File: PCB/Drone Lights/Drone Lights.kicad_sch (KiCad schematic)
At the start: 34 parts, among them J1 Proto Pin, J10 Prog_Connector, J11 Proto Pin, J12 Proto Pin, J13 Proto Pin, J14 Proto Pin, J2 Input, J3 Proto Pin, J4 Proto Pin, J5 Proto Pin, J6 Proto Pin, J7 Proto Pin, J8 Proto Pin, J9 Proto Pin, SW1 CT11024.3F160, SW2 CT11024.3F160, SW3 GF-123-0054, U1 ATTINY84A-PU

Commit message: Updated assembly guide
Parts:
- C1: Digikey No. (none) -> 445-1314-1-ND; MPN (none) -> C1608X7R1H104K080AA
- D1: Green MPN (none) -> XPEBGR-L1-0000-00F01; Red MPN (none) -> XPEBRD-L1-0000-00501; White MPN (none) -> XPEBWT-L1-0000-00C51
- D2, D3: MPN (none) -> B1911USD-20D000114U1930; Manufacturer PN B1911USD-20D000114U1930 -> (none)
- MOSFET1: Digikey No. (none) -> T2N7002BKLMCT-ND; MPN (none) -> T2N7002BK,LM
- R1: Digikey No. (none) -> P10.0HCT-ND; MPN (none) -> ERJ-3EKF10R0V
- R2, R3, R4: Digikey No. (none) -> RNCP0603FTD10K0CT-ND; MPN (none) -> RNCP0603FTD10K0
- R5: Digikey No. (none) -> 2019-RK73H1JRTTD4701FCT-ND; MPN (none) -> RK73H1JRTTD4701F
- SW1, SW2: Digikey No. (none) -> 2449-CT11024.3F160-ND; MPN (none) -> CT11024.3F160
- SW3: Digikey No. (none) -> CWI333-ND; MPN (none) -> GF-123-0054
- U1: Digikey No. (none) -> ATTINY84A-PU-ND; MPN (none) -> ATTINY84A-PU
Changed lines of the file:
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@@
+      (effects (font (size 1.27 1.27)) hide)
+    )
+    (property "Green MPN" "XPEBGR-L1-0000-00F01" (id 4) (at 35.56 74.295 0)
+      (effects (font (size 1.27 1.27)) hide)
+    )
+    (property "White MPN" "XPEBWT-L1-0000-00C51" (id 5) (at 35.56 74.295 0)
+      (effects (font (size 1.27 1.27)) hide)
+    )
+    (property "Red MPN" "XPEBRD-L1-0000-00501" (id 6) (at 35.56 74.295 0)
       (effects (font (size 1.27 1.27)) hide)
     )
@@
     )
     (property "Datasheet" "" (id 3) (at 46.99 69.215 0)
-      (effects (font (size 1.524 1.524)))
+      (effects (font (size 1.524 1.524)) hide)
+    )
+    (property "Digikey No." "T2N7002BKLMCT-ND" (id 4) (at 46.99 69.215 0)
+      (effects (font (size 1.27 1.27)) hide)
+    )
+    (property "MPN" "T2N7002BK,LM" (id 5) (at 46.99 69.215 0)
+      (effects (font (size 1.27 1.27)) hide)
     )
     (pin "1")
@@
       (effects (font (size 1.27 1.27)) hide)
     )
+    (property "Digikey No." "P10.0HCT-ND" (id 4) (at 42.545 74.295 90)
+      (effects (font (size 1.27 1.27)) hide)
+    )
+    (property "MPN" "ERJ-3EKF10R0V" (id 5) (at 42.545 74.295 90)
+      (effects (font (size 1.27 1.27)) hide)
+    )
     (pin "1")
     (pin "2")
@@
       (effects (font (size 1.27 1.27)) hide)
     )
+    (property "Digikey No." "RNCP0603FTD10K0CT-ND" (id 4) (at 218.44 66.04 90)
+      (effects (font (size 1.27 1.27)) hide)
+    )
+    (property "MPN" "RNCP0603FTD10K0" (id 5) (at 218.44 66.04 90)
+      (effects (font (size 1.27 1.27)) hide)
+    )
     (pin "1")
     (pin "2")
@@
       (effects (font (size 1.27 1.27)) hide)
     )
+    (property "Digikey No." "445-1314-1-ND" (id 4) (at 116.205 61.595 0)
+      (effects (font (size 1.27 1.27)) hide)
+    )
+    (property "MPN" "C1608X7R1H104K080AA" (id 5) (at 116.205 61.595 0)
+      (effects (font (size 1.27 1.27)) hide)
+    )
     (pin "1")
     (pin "2")
@@
     (property "Datasheet" "" (id 3) (at 46.99 121.285 0)
       (effects (font (size 1.524 1.524)))
+    )
+    (property "Digikey No." "2449-CT11024.3F160-ND" (id 4) (at 46.99 121.285 0)
+      (effects (font (size 1.27 1.27)) hide)
+    )
+    (property "MPN" "CT11024.3F160" (id 5) (at 46.99 121.285 0)
+      (effects (font (size 1.27 1.27)) hide)
     )
     (pin "1")
@@
       (effects (font (size 1.27 1.27)) hide)
     )
+    (property "Digikey No." "2019-RK73H1JRTTD4701FCT-ND" (id 4) (at 232.41 101.6 90)
+      (effects (font (size 1.27 1.27)) hide)
+    )
+    (property "MPN" "RK73H1JRTTD4701F" (id 5) (at 232.41 101.6 90)
+      (effects (font (size 1.27 1.27)) hide)
+    )
     (pin "1")
     (pin "2")
@@
       (effects (font (size 1.27 1.27)) hide)
     )
-    (property "Manufacturer PN" "B1911USD-20D000114U1930" (id 5) (at 248.92 66.04 0)
+    (property "MPN" "B1911USD-20D000114U1930" (id 5) (at 248.92 66.04 0)
       (effects (font (size 1.27 1.27)) hide)
     )
@@
       (effects (font (size 1.27 1.27)) hide)
     )
+    (property "Digikey No." "RNCP0603FTD10K0CT-ND" (id 4) (at 80.01 126.365 90)
+      (effects (font (size 1.27 1.27)) hide)
+    )
+    (property "MPN" "RNCP0603FTD10K0" (id 5) (at 80.01 126.365 90)
+      (effects (font (size 1.27 1.27)) hide)
+    )
     (pin "1")
     (pin "2")
@@
       (effects (font (size 1.27 1.27)) hide)
     )
+    (property "Digikey No." "RNCP0603FTD10K0CT-ND" (id 4) (at 80.01 109.22 90)
+      (effects (font (size 1.27 1.27)) hide)
+    )
+    (property "MPN" "RNCP0603FTD10K0" (id 5) (at 80.01 109.22 90)
+      (effects (font (size 1.27 1.27)) hide)
+    )
     (pin "1")
     (pin "2")
@@
     )
     (property "Datasheet" "" (id 3) (at 62.23 141.605 0)
-      (effects (font (size 1.524 1.524)))
+      (effects (font (size 1.524 1.524)) hide)
+    )
+    (property "Digikey No." "CWI333-ND" (id 4) (at 62.23 141.605 0)
+      (effects (font (size 1.27 1.27)) hide)
+    )
+    (property "MPN" "GF-123-0054" (id 5) (at 62.23 141.605 0)
+      (effects (font (size 1.27 1.27)) hide)
     )
     (pin "1")
@@
       (effects (font (size 1.27 1.27)) hide)
     )
-    (property "Manufacturer PN" "B1911USD-20D000114U1930" (id 5) (at 240.665 101.6 0)
+    (property "MPN" "B1911USD-20D000114U1930" (id 5) (at 240.665 101.6 0)
       (effects (font (size 1.27 1.27)) hide)
     )
@@
     )
     (property "Datasheet" "" (id 3) (at 46.99 104.14 0)
-      (effects (font (size 1.524 1.524)))
+      (effects (font (size 1.524 1.524)) hide)
+    )
+    (property "Digikey No." "2449-CT11024.3F160-ND" (id 4) (at 46.99 104.14 0)
+      (effects (font (size 1.27 1.27)) hide)
+    )
+    (property "MPN" "CT11024.3F160" (id 5) (at 46.99 104.14 0)
+      (effects (font (size 1.27 1.27)) hide)
     )
     (pin "1")
@@
       (effects (font (size 1.524 1.524)) hide)
     )
-    (property "Datasheet" "" (id 3) (at 121.92 65.405 0)
-      (effects (font (size 1.524 1.524)))
-    )
-    (pin "1")
+    (property "Datasheet" "https://www.digikey.ca/en/products/detail/microchip-technology/ATTINY84A-PU/2774082" (id 3) (at 121.92 65.405 0)
+      (effects (font (size 1.524 1.524)) hide)
+    )
+    (property "Digikey No." "ATTINY84A-PU-ND" (id 4) (at 121.92 65.405 0)
+      (effects (font (size 1.27 1.27)) hide)
+    )
+    (property "MPN" "ATTINY84A-PU" (id 5) (at 121.92 65.405 0)
+      (effects (font (size 1.27 1.27)) hide)
+    )
+    (pin "1")

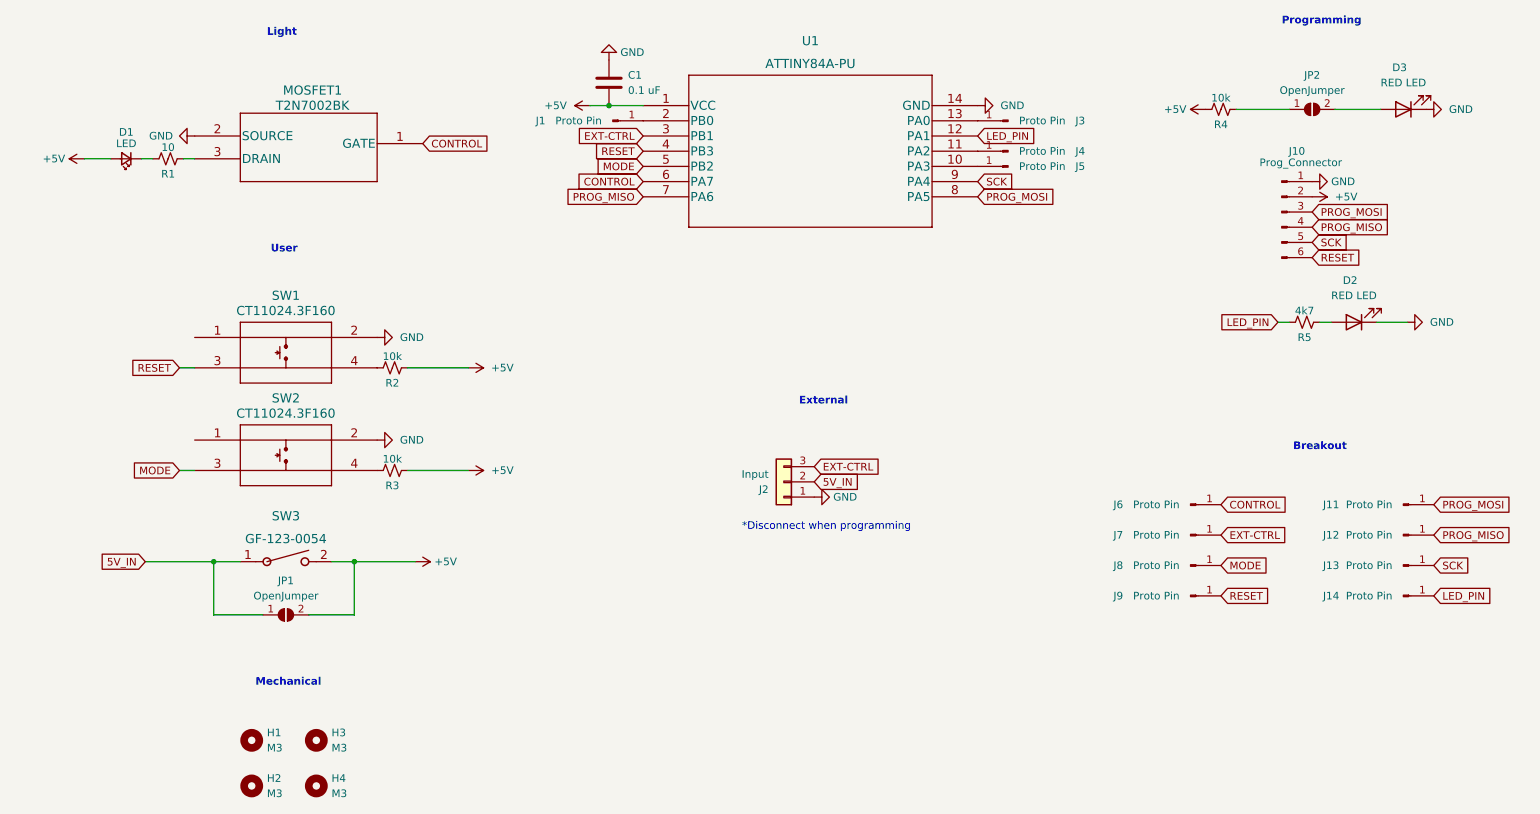
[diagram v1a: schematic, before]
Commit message: Updated with local copy
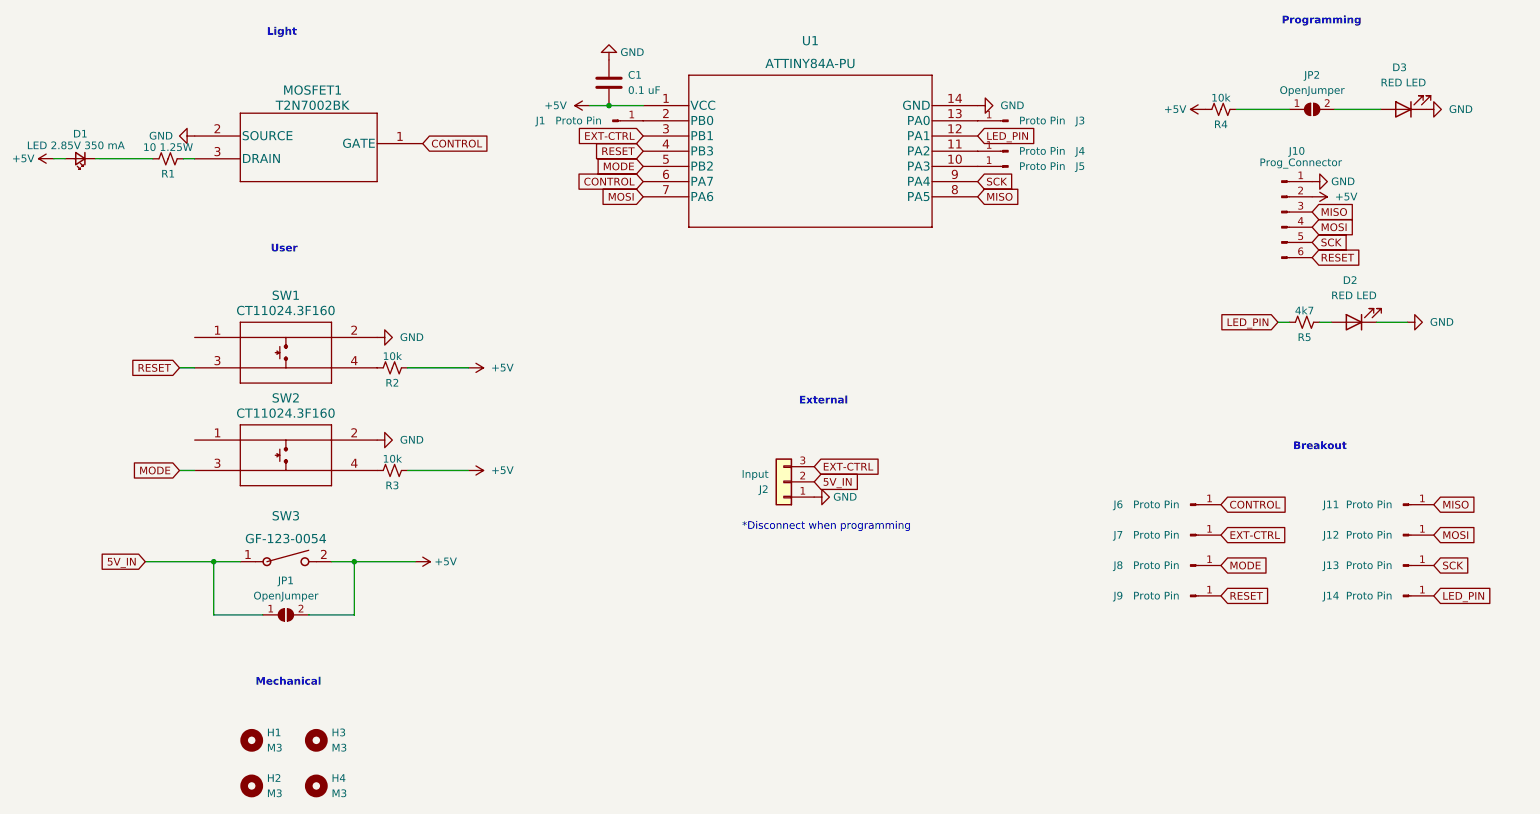
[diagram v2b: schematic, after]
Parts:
- D1: value LED -> LED 2.85V 350 mA
- R1: value 10 -> 10 1.25W; Digikey No. P10.0HCT-ND -> A130636CT-ND; MPN ERJ-3EKF10R0V -> CRGP2010F10R
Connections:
- net PROG_MISO renamed MOSI
- net PROG_MOSI renamed MISO
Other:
- moved on the sheet: D1
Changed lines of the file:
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@@
   (title_block
     (title "Drone Lights")
-    (rev "A")
+    (rev "B")
     (company "Designer: Sonia Wong")
   )
@@
     (stroke (width 0) (type default) (color 0 0 0 0))
   )
-  (wire (pts (xy 28.575 74.295) (xy 33.02 74.295))
+  (wire (pts (xy 23.4472 74.2694) (xy 25.3427 74.2694))
     (stroke (width 0) (type default) (color 0 0 0 0))
   )
@@
     (stroke (width 0) (type default) (color 0 0 0 0))
   )
-  (wire (pts (xy 38.1 74.295) (xy 40.005 74.295))
+  (wire (pts (xy 30.4227 74.2694) (xy 40.005 74.295))
     (stroke (width 0) (type default) (color 0 0 0 0))
   )
@@
     )
   )
-  (global_label "PROG_MOSI" (shape input) (at 177.8 80.645 0) (fields_autoplaced)
-    (effects (font (size 1.27 1.27)) (justify left))
-    (property "Intersheet References" "${INTERSHEET_REFS}" (id 0) (at 190.9174 80.5656 0)
+  (global_label "MISO" (shape input) (at 177.8 80.645 0) (fields_autoplaced)
+    (effects (font (size 1.27 1.27)) (justify left))
+    (property "Intersheet References" "${INTERSHEET_REFS}" (id 0) (at 184.8093 80.5656 0)
       (effects (font (size 1.27 1.27)) (justify left) hide)
     )
@@
     )
   )
-  (global_label "PROG_MISO" (shape input) (at 121.92 80.645 180) (fields_autoplaced)
+  (global_label "MOSI" (shape input) (at 121.92 80.645 180) (fields_autoplaced)
     (effects (font (size 1.27 1.27)) (justify right))
-    (property "Intersheet References" "${INTERSHEET_REFS}" (id 0) (at 108.8026 80.7244 0)
+    (property "Intersheet References" "${INTERSHEET_REFS}" (id 0) (at 114.9107 80.5656 0)
       (effects (font (size 1.27 1.27)) (justify right) hide)
     )
   )
-  (global_label "PROG_MOSI" (shape input) (at 233.68 83.185 0) (fields_autoplaced)
-    (effects (font (size 1.27 1.27)) (justify left))
-    (property "Intersheet References" "${INTERSHEET_REFS}" (id 0) (at 246.7974 83.1056 0)
+  (global_label "MISO" (shape input) (at 233.68 83.185 0) (fields_autoplaced)
+    (effects (font (size 1.27 1.27)) (justify left))
+    (property "Intersheet References" "${INTERSHEET_REFS}" (id 0) (at 240.6893 83.1056 0)
       (effects (font (size 1.27 1.27)) (justify left) hide)
     )
@@
     )
   )
-  (global_label "PROG_MOSI" (shape input) (at 254 132.08 0) (fields_autoplaced)
-    (effects (font (size 1.27 1.27)) (justify left))
-    (property "Intersheet References" "${INTERSHEET_REFS}" (id 0) (at 267.1174 132.0006 0)
+  (global_label "MISO" (shape input) (at 254 132.08 0) (fields_autoplaced)
+    (effects (font (size 1.27 1.27)) (justify left))
+    (property "Intersheet References" "${INTERSHEET_REFS}" (id 0) (at 261.0093 132.0006 0)
       (effects (font (size 1.27 1.27)) (justify left) hide)
     )
@@
     )
   )
-  (global_label "PROG_MISO" (shape input) (at 233.68 85.725 0) (fields_autoplaced)
-    (effects (font (size 1.27 1.27)) (justify left))
-    (property "Intersheet References" "${INTERSHEET_REFS}" (id 0) (at 246.7974 85.6456 0)
+  (global_label "MOSI" (shape input) (at 233.68 85.725 0) (fields_autoplaced)
+    (effects (font (size 1.27 1.27)) (justify left))
+    (property "Intersheet References" "${INTERSHEET_REFS}" (id 0) (at 240.6893 85.6456 0)
       (effects (font (size 1.27 1.27)) (justify left) hide)
     )
@@
     )
   )
-  (global_label "PROG_MISO" (shape input) (at 254 137.16 0) (fields_autoplaced)
-    (effects (font (size 1.27 1.27)) (justify left))
-    (property "Intersheet References" "${INTERSHEET_REFS}" (id 0) (at 267.1174 137.0806 0)
+  (global_label "MOSI" (shape input) (at 254 137.16 0) (fields_autoplaced)
+    (effects (font (size 1.27 1.27)) (justify left))
+    (property "Intersheet References" "${INTERSHEET_REFS}" (id 0) (at 261.0093 137.0806 0)
       (effects (font (size 1.27 1.27)) (justify left) hide)
     )
@@
     (pin "1")
   )
-  (symbol (lib_id "Device:LED_Small") (at 35.56 74.295 180) (unit 1)
-    (in_bom yes) (on_board yes)
-    (property "Reference" "D1" (id 0) (at 35.56 69.85 0))
-    (property "Value" "LED" (id 1) (at 35.56 71.755 0))
-    (property "Footprint" "XLAMP:XLAMP_LED_XPE2" (id 2) (at 35.56 74.295 90)
-      (effects (font (size 1.27 1.27)) hide)
-    )
-    (property "Datasheet" "~" (id 3) (at 35.56 74.295 90)
-      (effects (font (size 1.27 1.27)) hide)
-    )
-    (property "Green MPN" "XPEBGR-L1-0000-00F01" (id 4) (at 35.56 74.295 0)
-      (effects (font (size 1.27 1.27)) hide)
-    )
-    (property "White MPN" "XPEBWT-L1-0000-00C51" (id 5) (at 35.56 74.295 0)
-      (effects (font (size 1.27 1.27)) hide)
-    )
-    (property "Red MPN" "XPEBRD-L1-0000-00501" (id 6) (at 35.56 74.295 0)
+  (symbol (lib_id "Device:LED_Small") (at 27.8827 74.2694 180) (unit 1)
+    (in_bom yes) (on_board yes)
+    (property "Reference" "D1" (id 0) (at 27.8827 70.1451 0))
+    (property "Value" "LED 2.85V 350 mA" (id 1) (at 27.1328 72.0948 0))
+    (property "Footprint" "XLAMP:XLAMP_LED_XPE2" (id 2) (at 27.8827 74.2694 90)
+      (effects (font (size 1.27 1.27)) hide)
+    )
+    (property "Datasheet" "~" (id 3) (at 27.8827 74.2694 90)
+      (effects (font (size 1.27 1.27)) hide)
+    )
+    (property "Green MPN" "XPEBGR-L1-0000-00F01" (id 4) (at 27.8827 74.2694 0)
+      (effects (font (size 1.27 1.27)) hide)
+    )
+    (property "White MPN" "XPEBWT-L1-0000-00C51" (id 5) (at 27.8827 74.2694 0)
+      (effects (font (size 1.27 1.27)) hide)
+    )
+    (property "Red MPN" "XPEBRD-L1-0000-00501" (id 6) (at 27.8827 74.2694 0)
       (effects (font (size 1.27 1.27)) hide)
     )
@@
     (in_bom yes) (on_board yes)
     (property "Reference" "R1" (id 0) (at 42.545 76.835 90))
-    (property "Value" "10" (id 1) (at 42.545 72.39 90))
+    (property "Value" "10 1.25W" (id 1) (at 42.545 72.39 90))
     (property "Footprint" "Resistor_SMD:R_0603_1608Metric_Pad0.98x0.95mm_HandSolder" (id 2) (at 42.545 74.295 0)
       (effects (font (size 1.27 1.27)) hide)
@@
       (effects (font (size 1.27 1.27)) hide)
     )
-    (property "Digikey No." "P10.0HCT-ND" (id 4) (at 42.545 74.295 90)
-      (effects (font (size 1.27 1.27)) hide)
-    )
-    (property "MPN" "ERJ-3EKF10R0V" (id 5) (at 42.545 74.295 90)
+    (property "Digikey No." "A130636CT-ND" (id 4) (at 42.545 74.295 90)
+      (effects (font (size 1.27 1.27)) hide)
+    )
+    (property "MPN" "CRGP2010F10R" (id 5) (at 42.545 74.295 90)
       (effects (font (size 1.27 1.27)) hide)
     )
@@
     (pin "1")
   )
-  (symbol (lib_id "power:+5V") (at 28.575 74.295 90) (unit 1)
-    (in_bom yes) (on_board yes)
-    (property "Reference" "#PWR01" (id 0) (at 32.385 74.295 0)
-      (effects (font (size 1.27 1.27)) hide)
-    )
-    (property "Value" "+5V" (id 1) (at 21.59 74.295 90)
-      (effects (font (size 1.27 1.27)) (justify right))
-    )
-    (property "Footprint" "" (id 2) (at 28.575 74.295 0)
-      (effects (font (size 1.27 1.27)) hide)
-    )
-    (property "Datasheet" "" (id 3) (at 28.575 74.295 0)
+  (symbol (lib_id "power:+5V") (at 23.4472 74.2694 90) (unit 1)
+    (in_bom yes) (on_board yes)
+    (property "Reference" "#PWR01" (id 0) (at 27.2572 74.2694 0)
+      (effects (font (size 1.27 1.27)) hide)
+    )
+    (property "Value" "+5V" (id 1) (at 16.4622 74.2694 90)
+      (effects (font (size 1.27 1.27)) (justify right))
+    )
+    (property "Footprint" "" (id 2) (at 23.4472 74.2694 0)
+      (effects (font (size 1.27 1.27)) hide)
+    )
+    (property "Datasheet" "" (id 3) (at 23.4472 74.2694 0)
       (effects (font (size 1.27 1.27)) hide)
     )
@@
     )
     (path "/15ec28ff-48b3-42c7-a3dd-59b34880f0af"
-      (reference "D1") (unit 1) (value "LED") (footprint "XLAMP:XLAMP_LED_XPE2")
+      (reference "D1") (unit 1) (value "LED 2.85V 350 mA") (footprint "XLAMP:XLAMP_LED_XPE2")
     )
     (path "/e2e0e042-ddec-41d3-b4e5-fb1f6f7261f1"
@@
     )
     (path "/41f01e22-aaf1-4c89-9c10-b9e09a4f5396"
-      (reference "R1") (unit 1) (value "10") (footprint "Resistor_SMD:R_0603_1608Metric_Pad0.98x0.95mm_HandSolder")
+      (reference "R1") (unit 1) (value "10 1.25W") (footprint "Resistor_SMD:R_0603_1608Metric_Pad0.98x0.95mm_HandSolder")
     )
     (path "/ca2e86ab-486d-4490-aec7-75750b67e728"
